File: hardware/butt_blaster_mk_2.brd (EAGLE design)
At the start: 44 x 40 mm, 23 parts, among them IC1 HV9922

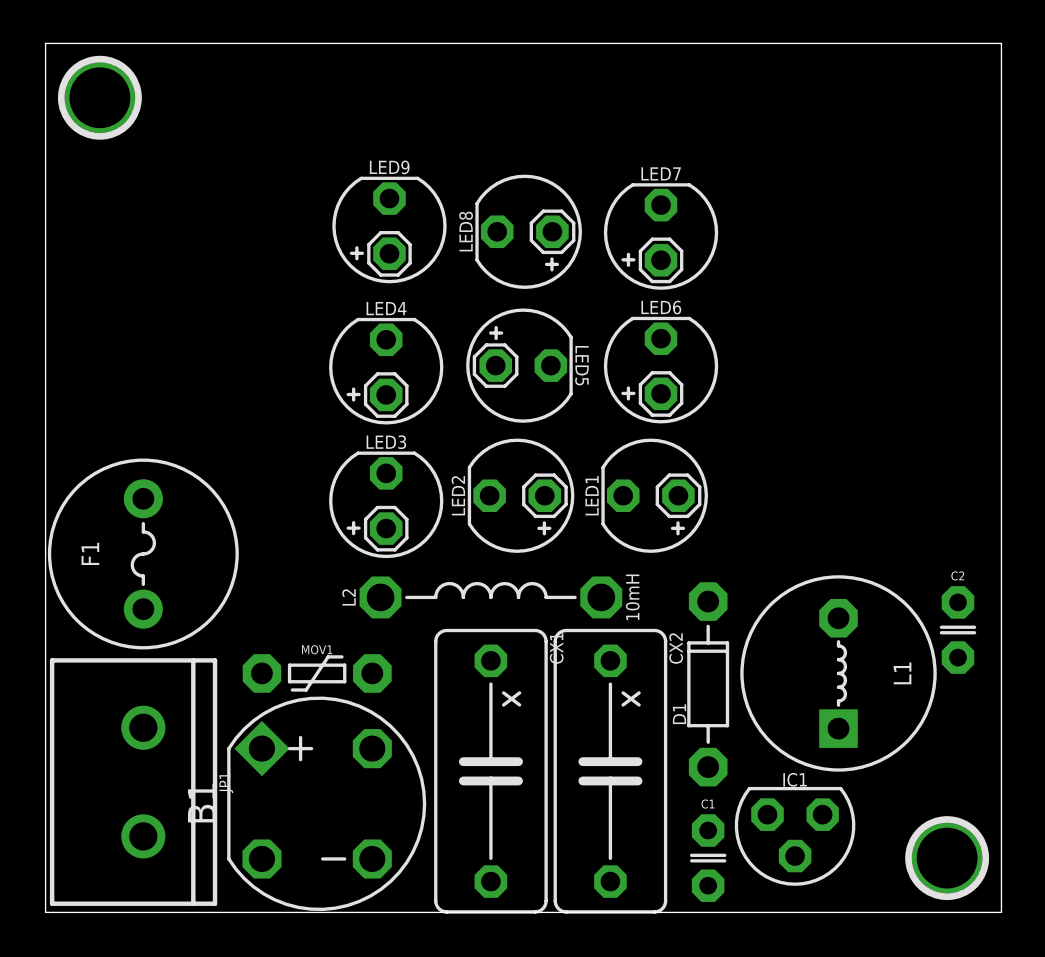
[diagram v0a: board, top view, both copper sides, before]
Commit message: butts
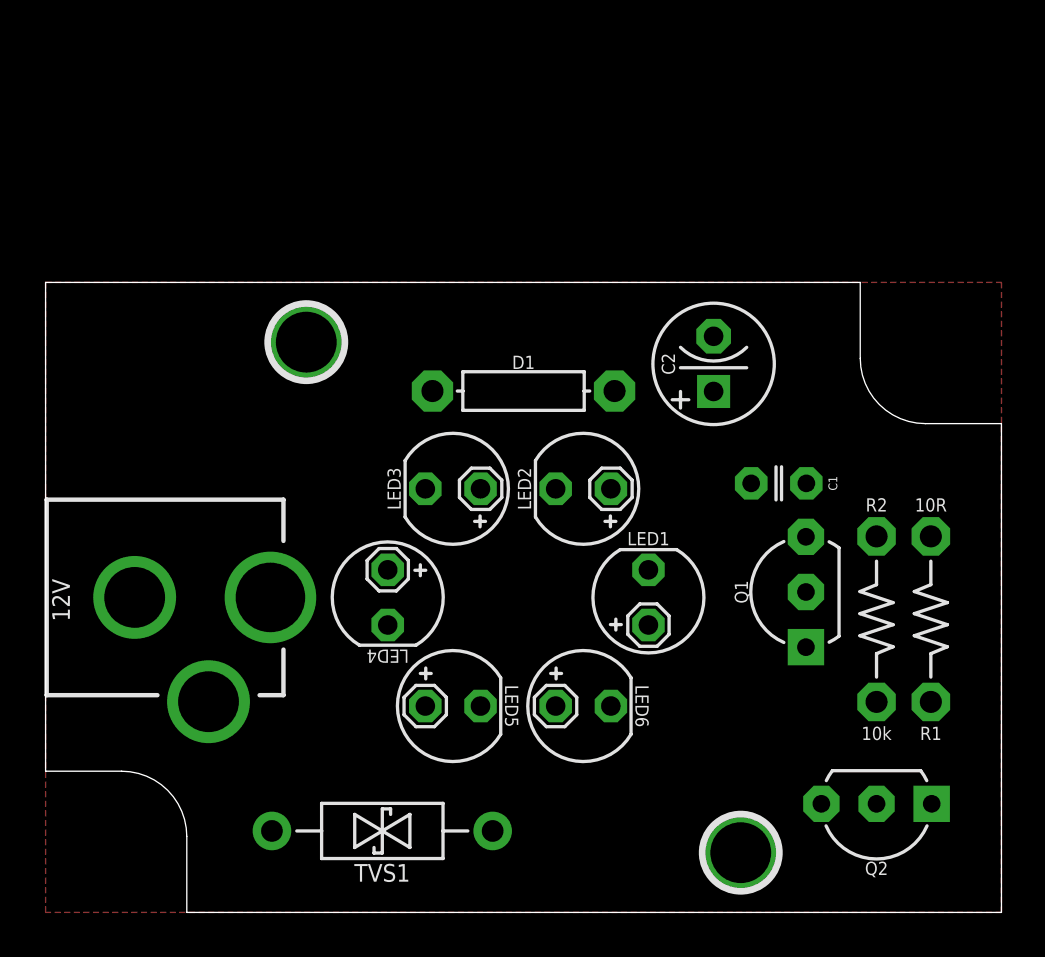
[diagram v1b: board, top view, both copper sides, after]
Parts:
- removed B1: (no value), A_butts:RB1A-NOSUCK
- removed CX1, CX2: 0.1uF, A_butts:XC10B5
- removed F1: 250mA(?), A_butts:TR5
- removed IC1: HV9922, A_butts:TO-92
- removed JP1: M025MM, A_butts:SCREWTERMINAL-5MM-2
- removed L1: 10mH, A_butts:RLB0912
- removed L2: 10mH, A_butts:INDUCTOR-AXIAL-PTH-10.16MM
- removed LED7, LED8, LED9: LED5MM_SHORTPADS, A_butts:LED5MM_SHORTPADS
- removed MOV1: (no value), A_butts:VAR-5.08MM-PTH
- added 12V: (no value), A_butts:DCJACK_2MM_PTH
- added Q1: 2N3904, A_butts:TO-92-AMMO
- added Q2: 2N7000, A_butts:TO-92-AMMO
- added R1: 10R, A_butts:RESISTOR-AXIAL-PTH-7.68MM
- added R2: 10k, A_butts:RESISTOR-AXIAL-PTH-7.68MM
- added TVS1: (no value), A_butts:DO-41-TVS
- C2: device A_butts:C025-024X044 -> A_butts:E2,5-6
- D1: device A_butts:DIODE-7.68MM -> A_butts:DIODE-8.38MM
- moved C1 17.6 mm to (33.8, 19.8), turned to 180 degrees
- moved C2 16.6 mm to (30.8, 25.2), turned to 90 degrees
- moved LED6 16.0 mm to (24.8, 9.50), turned to 0 degrees
- moved LED5 16.0 mm to (18.8, 9.50)
- moved D1 16.0 mm to (22.0, 24.0), turned to 0 degrees
- moved H1 14.7 mm to (12.0, 26.2)
- moved LED4 10.6 mm to (15.8, 14.5), turned to 270 degrees
- moved H2 9.50 mm to (32.0, 2.75)
- moved LED1 4.68 mm to (27.8, 14.5), turned to 90 degrees
- moved LED3 3.12 mm to (18.8, 19.5), turned to 180 degrees
- moved LED2 3.06 mm to (24.8, 19.5)
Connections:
- removed net AC(L): F1.1, JP1.2
- removed net AC(N): B1.AC2, JP1.1, MOV1.1
- removed net N$10 (its old number): D1.A, IC1.1, L1.1
- removed net N$11: C2.1, CX2.1, D1.K, L2.P$2, LED1.A
- removed net N$13: B1.+, CX1.1, L2.P$1
- removed net N$14: C1.1, IC1.3
- removed net N$9: C2.2, L1.2, LED9.K
- new net VCC: C1.1, C2.+, D1.K, LED1.A, Q1.3, R2.P$1
- net GND: now also 12V.BRK, 12V.GND, C2.-, Q1.1, R1.P$2, TVS1.P$1; no longer B1.-, CX1.2, CX2.2, IC1.2
- net N$12: now also 12V.PWR, D1.A, TVS1.P$2; no longer B1.AC1, F1.2, MOV1.2
- net N$6: now also Q1.2, Q2.1, R1.P$1; no longer LED6.K, LED7.A
- net N$7: now also LED6.K, Q2.3; no longer LED7.K, LED8.A
- net N$8: now also Q2.2, R2.P$2; no longer LED8.K, LED9.A
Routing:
- added copper zone on layer 1, net GND
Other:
- board size 44 x 40 mm -> 44 x 29 mm
